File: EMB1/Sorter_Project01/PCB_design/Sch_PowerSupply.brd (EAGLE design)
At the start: 69.5 x 79.3 mm, 13 parts, among them IC1 LM2574N-3.3, IC2 7812T, IC3 7806T

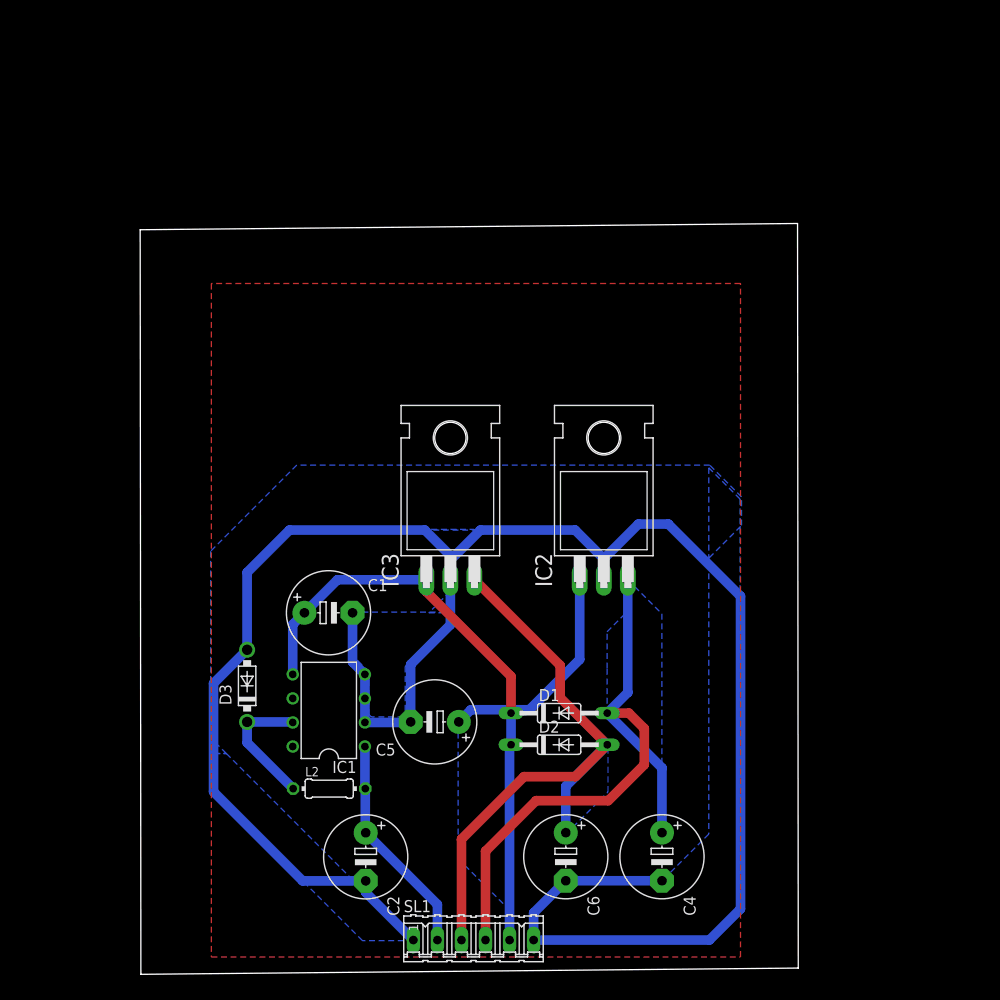
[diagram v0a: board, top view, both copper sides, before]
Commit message: brd update
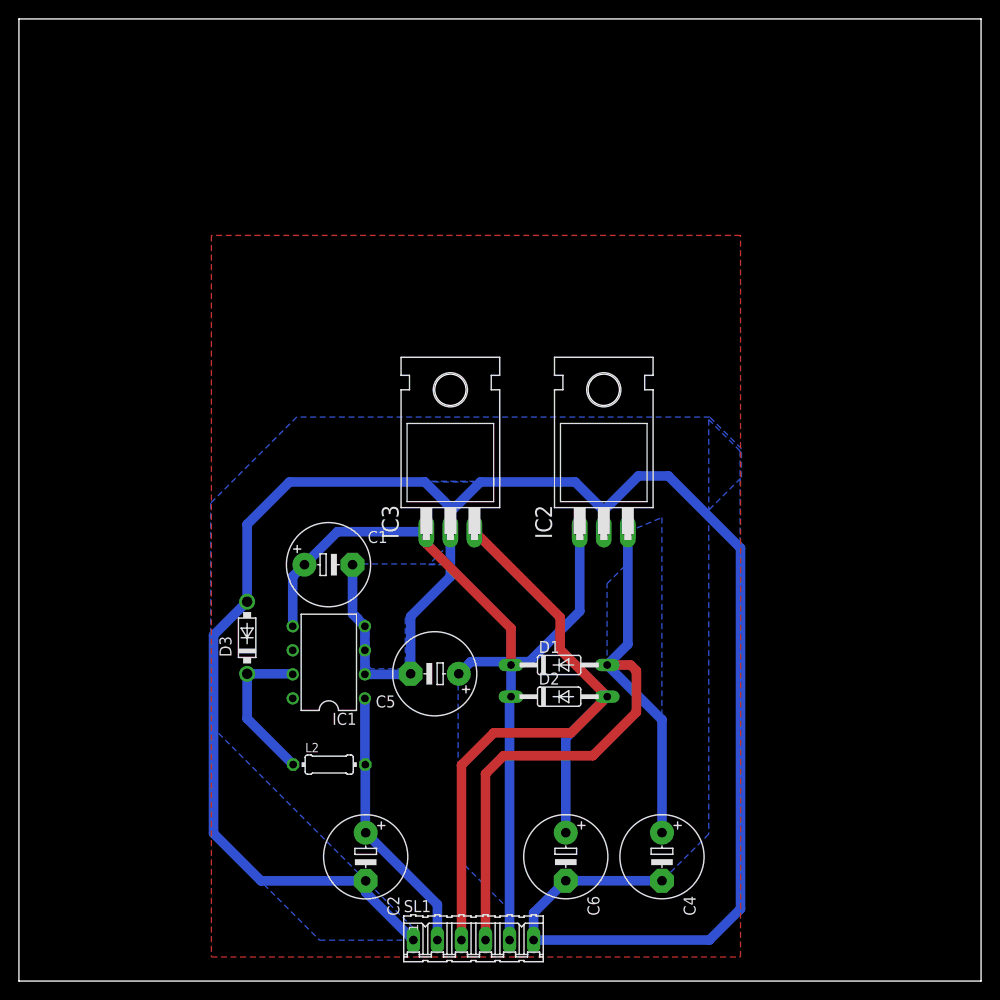
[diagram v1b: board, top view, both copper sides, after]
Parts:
- moved IC1 5.08 mm to (32.7, 33.7)
- moved C1 5.08 mm to (32.7, 44.0)
- moved C5 5.08 mm to (43.9, 32.4)
- moved D1 5.08 mm to (57.0, 33.4)
- moved D2 5.08 mm to (57.0, 30.0)
- moved D3 5.08 mm to (24.1, 36.3)
- moved IC2 5.08 mm to (61.8, 57.6)
- moved IC3 5.08 mm to (45.6, 57.6)
- moved L2 2.54 mm to (32.8, 22.9)
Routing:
- net GND: track 227.8 -> 240.5 mm
- net 6V: track 64.5 -> 75.7 mm
- net 12V: track 68.3 -> 79.0 mm
- net 5V: track 23.6 -> 28.7 mm
- net 15V: track 89.0 -> 94.1 mm
- net N$1: track 13.9 -> 16.4 mm
- removed copper zone on layer 16, net 6V
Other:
- board size 69.5 x 79.3 mm -> 101.6 x 101.6 mm
